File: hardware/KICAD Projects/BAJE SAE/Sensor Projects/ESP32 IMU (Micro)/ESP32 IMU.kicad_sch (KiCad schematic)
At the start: 4 parts, among them J1 Conn_01x02

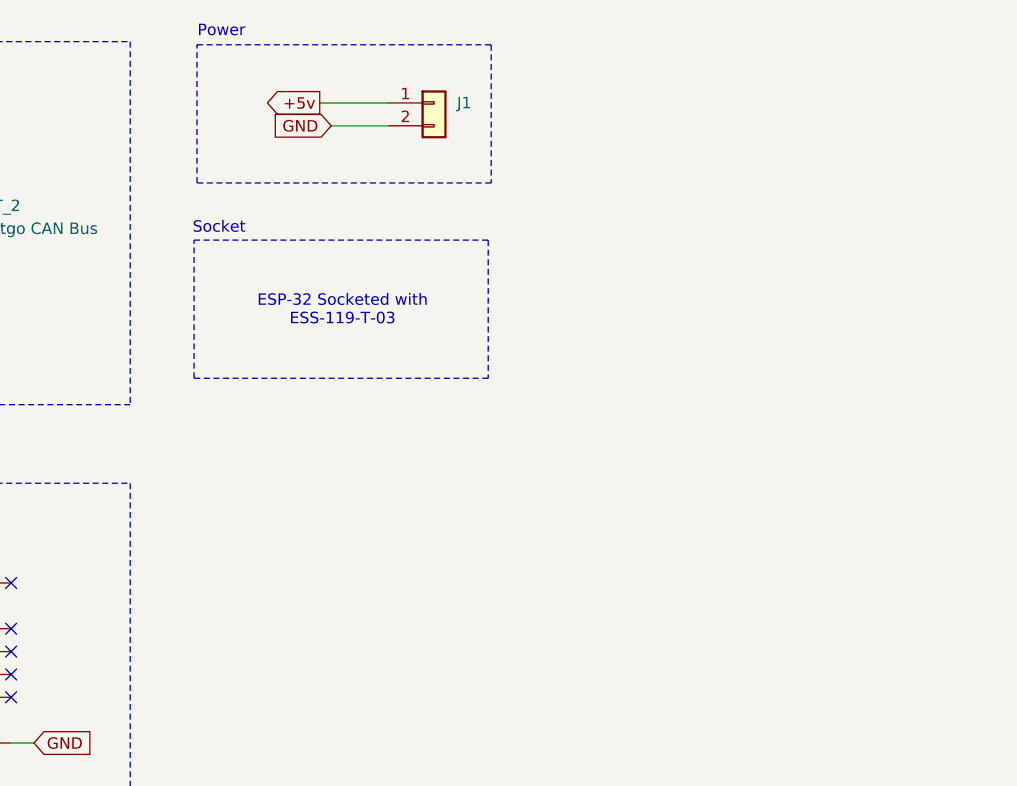
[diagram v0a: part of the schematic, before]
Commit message: Updates to IMU and Temp PCB
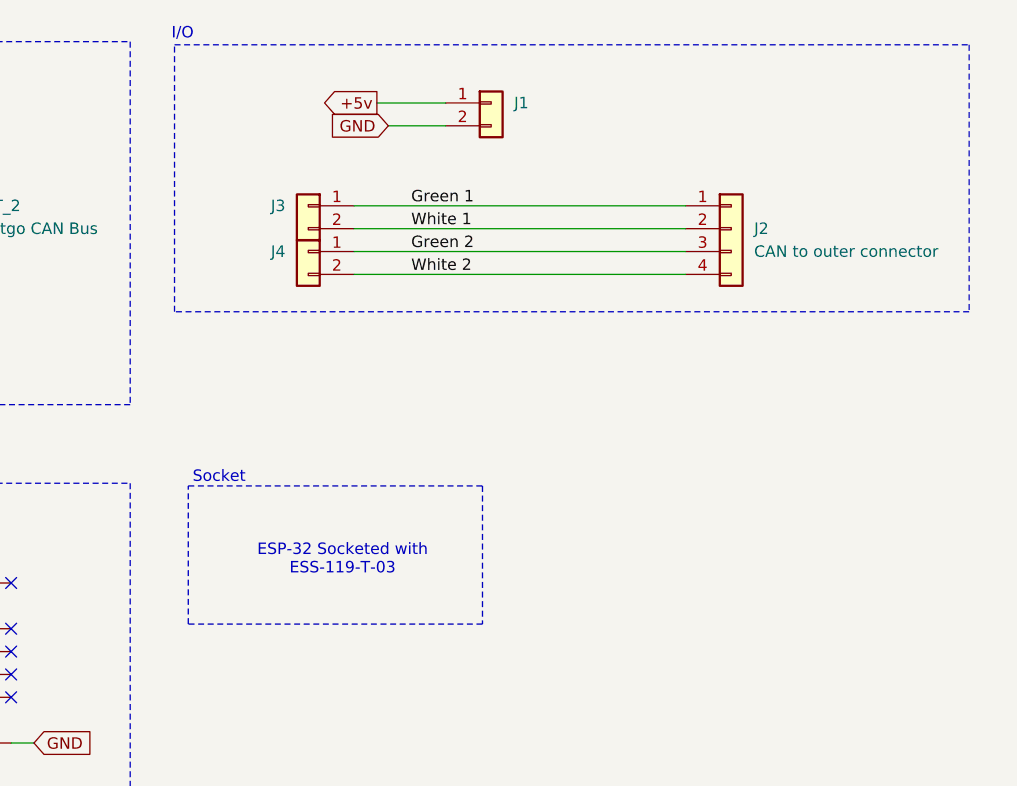
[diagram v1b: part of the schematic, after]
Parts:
- added J2: CAN to outer connector, Connector_Wire:SolderWire-0.1sqmm_1x04_P3.6mm_D0.4mm_OD1mm_Relief, symbol Connector_Generic:Conn_01x04
- added J3, J4: Conn_01x02, Connector_PinHeader_2.54mm:PinHeader_1x02_P2.54mm_Vertical, symbol Connector_Generic:Conn_01x02
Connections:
- new net Green 1: J2.1 (Pin_1), J3.1 (Pin_1)
- new net Green 2: J2.3 (Pin_3), J4.1 (Pin_1)
- new net White 1: J2.2 (Pin_2), J3.2 (Pin_2)
- new net White 2: J2.4 (Pin_4), J4.2 (Pin_2)
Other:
- note added: "I/O"
- note removed: "Power"
- moved on the sheet: J1

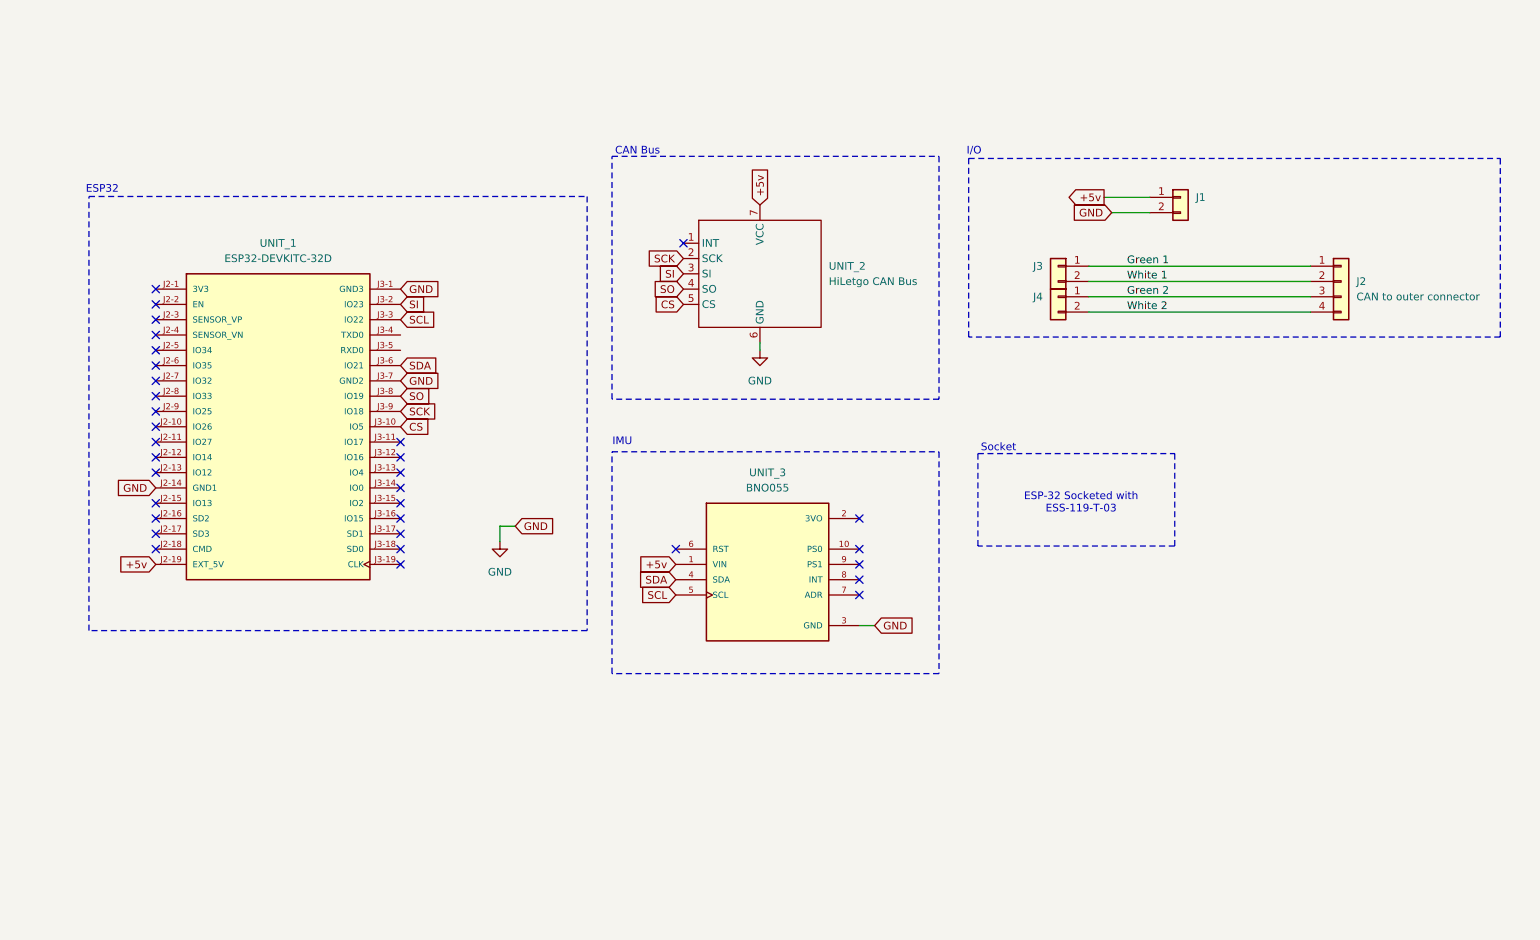
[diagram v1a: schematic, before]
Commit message: Updates to IMU and Temp.
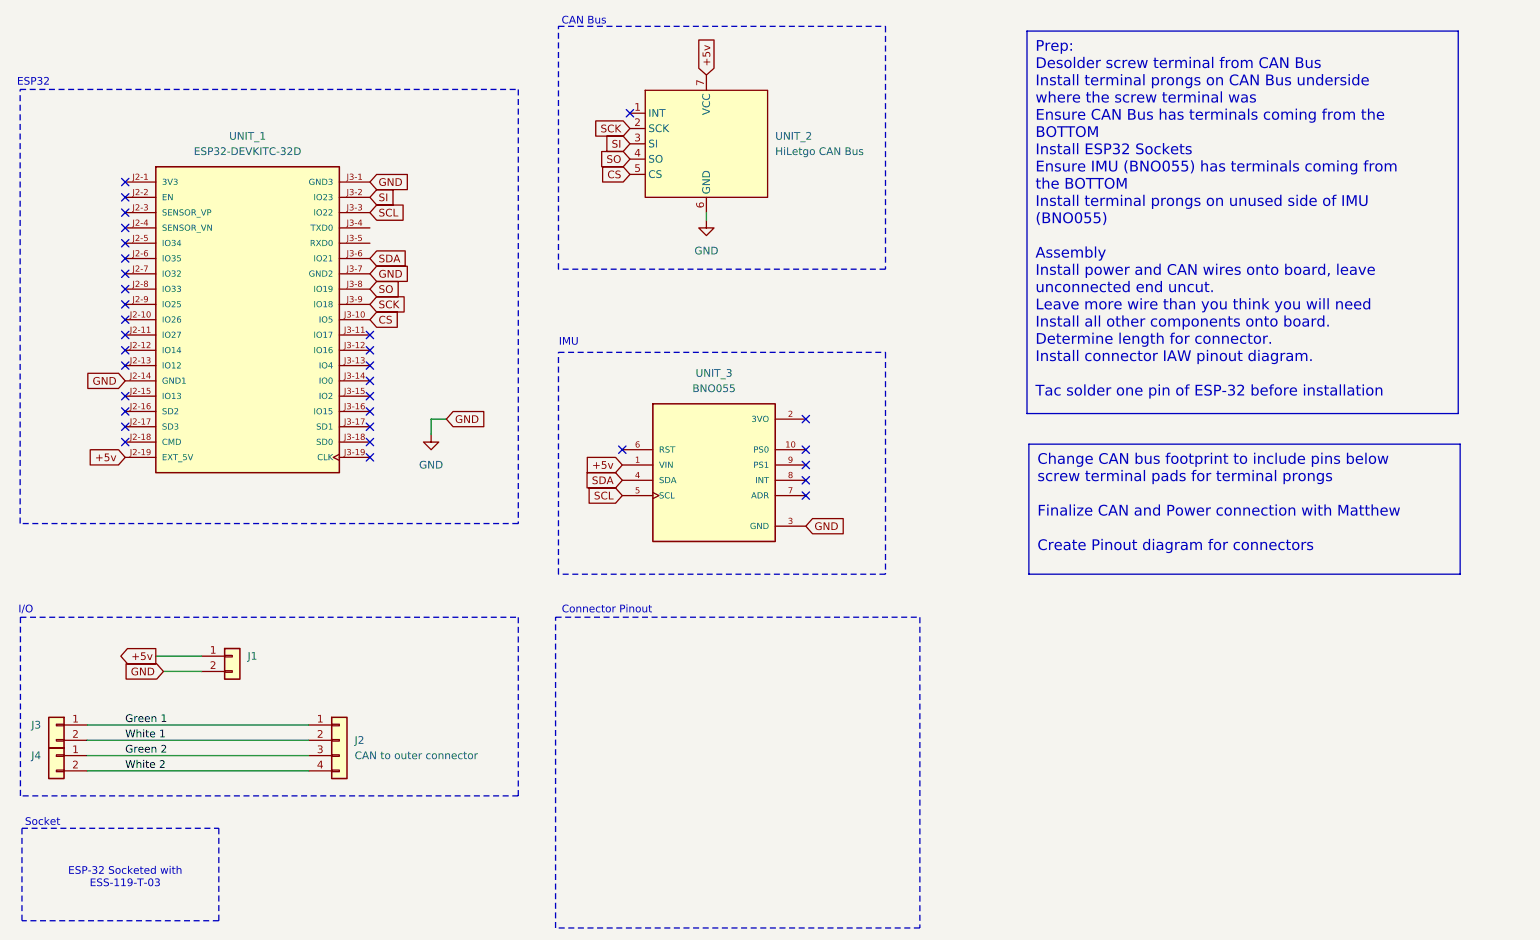
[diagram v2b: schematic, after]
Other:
- note added: "Connector Pinout"
- moved on the sheet: J1, J2, J3, J4, UNIT_1, UNIT_3
